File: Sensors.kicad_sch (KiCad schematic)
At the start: 13 parts, among them U16 TPRT9013-33, U17 ICM-42688-P, U18 BMP280, U19 INA230

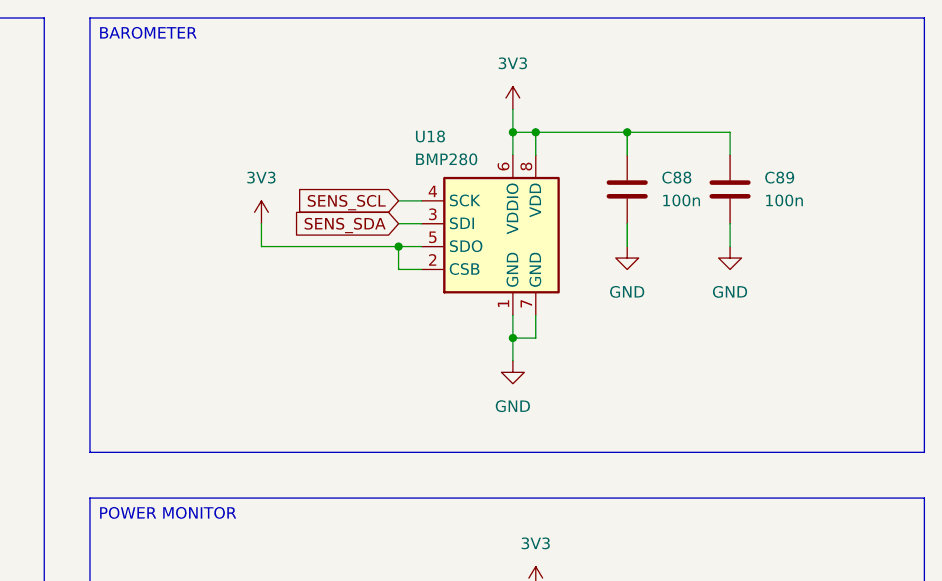
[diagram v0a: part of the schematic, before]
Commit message: MCU layout
Started the MCU layout.

TODO:
Check the previous iterations.
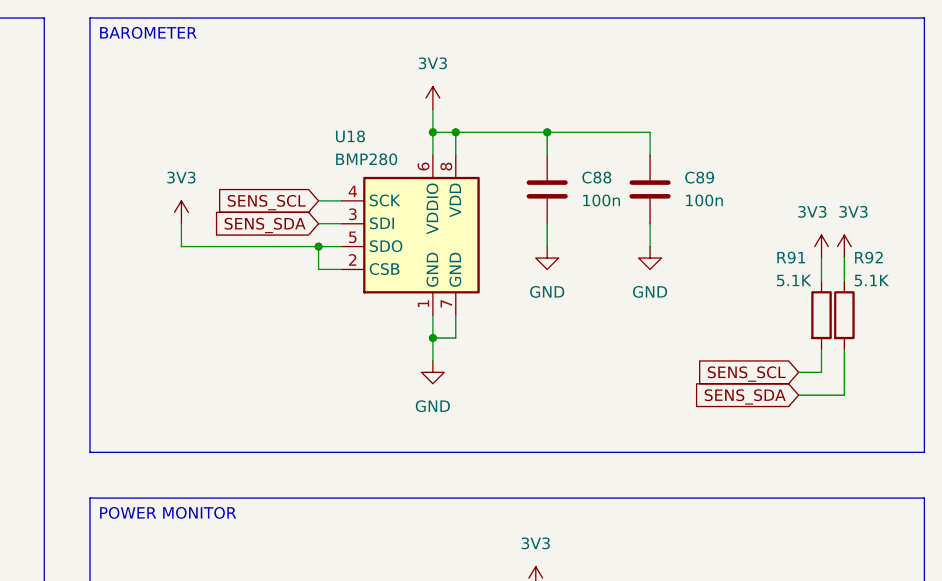
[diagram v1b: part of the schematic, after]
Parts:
- added R91, R92: 5.1K, Resistor_SMD:R_0603_1608Metric, symbol Device:R
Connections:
- net 3V3: now also R91.1, R92.1
- net SENS_SCL: now also R91.2
- net SENS_SDA: now also R92.2
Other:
- moved on the sheet: C88, C89, U18
